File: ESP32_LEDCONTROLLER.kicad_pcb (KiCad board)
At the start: 2 copper layers, 52.6 x 65.3 mm, 19 parts, among them J1 ST-04, J2 Screw_Terminal_01x04, J3 Screw_Terminal_01x04, J4 Screw_Terminal_01x04, J5 Screw_Terminal_01x04, U1 LM2576HVT-5, U2 ESP32-DEVKIT-V1

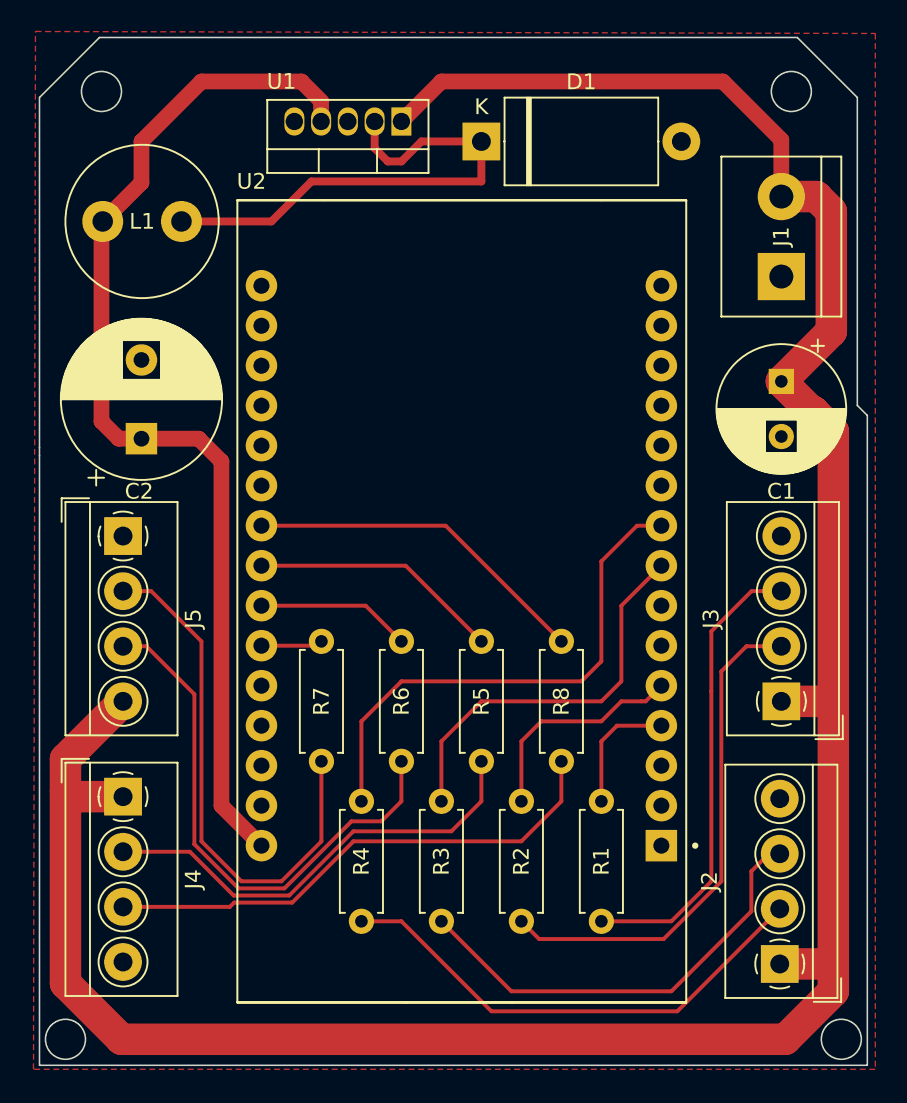
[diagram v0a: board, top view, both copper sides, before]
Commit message: graphics & shitposting
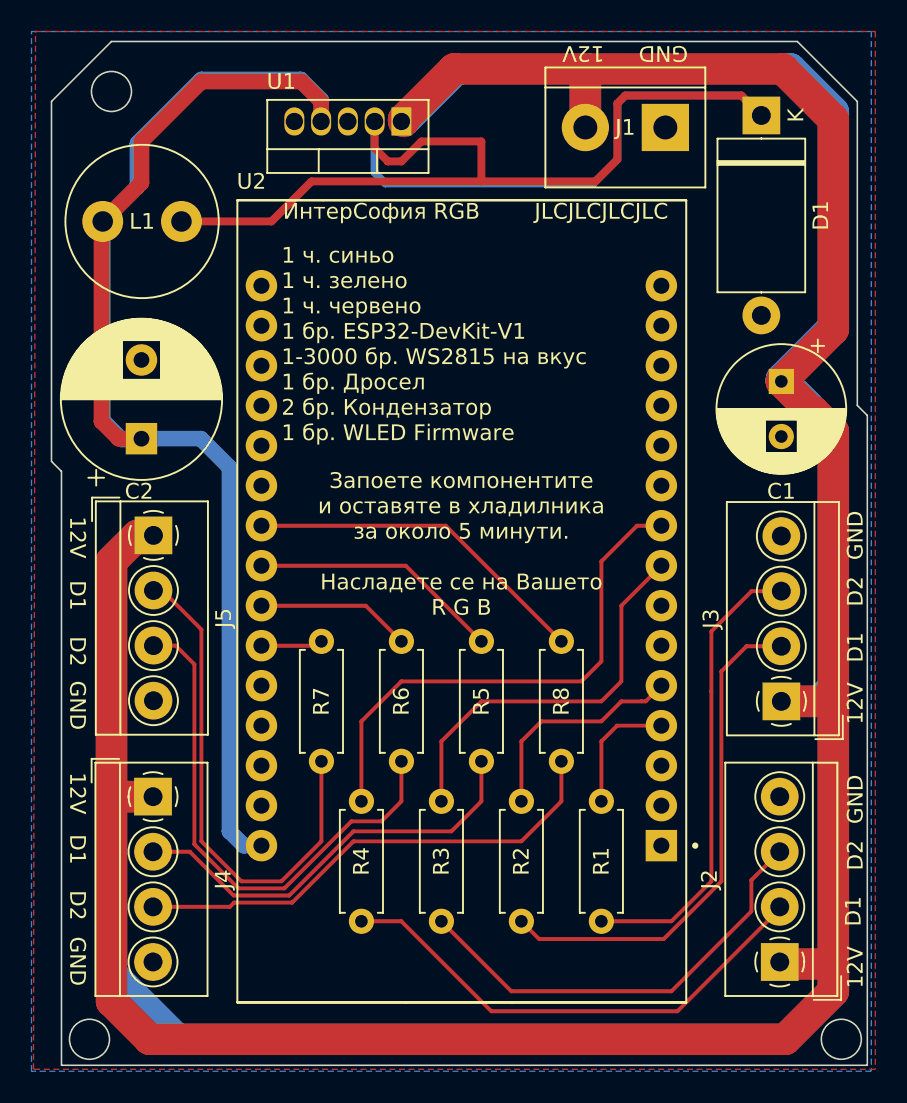
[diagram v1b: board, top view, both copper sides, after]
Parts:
- added G***: LOGO, table:intersofia-pcb-info_neg, B.Cu at (116.9, 121.8)
- moved D1 17.9 mm to (135.9, 94.9), turned to -90 degrees
- moved J1 12.0 mm to (129.8, 95.6), turned to 180 degrees
- moved J5 1.93 mm to (97.3, 121.5)
- moved J4 1.91 mm to (97.3, 138.1)
- moved J2 0.13 mm to (137.1, 148.6)
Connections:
- J5 pad 1: GND -> VSS
- J5 pad 4: VSS -> GND
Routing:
- net VSS: track 167.8 -> 361.2 mm
- net Net-(D1-Pad1): track 32.0 -> 87.5 mm
- net VCC: track 67.8 -> 105.3 mm
- net Net-(J4-Pad3): track 33.2 -> 31.3 mm
- net Net-(J4-Pad2): track 28.9 -> 27.0 mm
- net Net-(J5-Pad2): track 33.8 -> 32.3 mm
- net Net-(J5-Pad3): track 34.5 -> 33.7 mm
- added copper zone on B.Cu, net GND
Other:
- board size 52.6 x 65.3 mm -> 51.8 x 65 mm
- board text added: "1 ч. синьо 1 ч. зелено 1 ч. червено 1 бр. ESP32-DevKit-V1 1-3000 бр. WS2815 на вкус 1 бр. Дросел 2 бр. Кондензатор 1 бр. WLED Firmware"
- board text added: "12V"
- board text added: "D1"
- board text added: "D2"
- board text added: "GND"
- board text added: "JLCJLCJLCJLC"
- board text added: "Запоете компонентите и оставяте в хладилника за около 5 минути. Насладете се на Вашето R G B"
- board text added: "ИнтерСофия RGB"
